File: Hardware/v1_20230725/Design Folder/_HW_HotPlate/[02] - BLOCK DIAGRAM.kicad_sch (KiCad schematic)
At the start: 0 parts

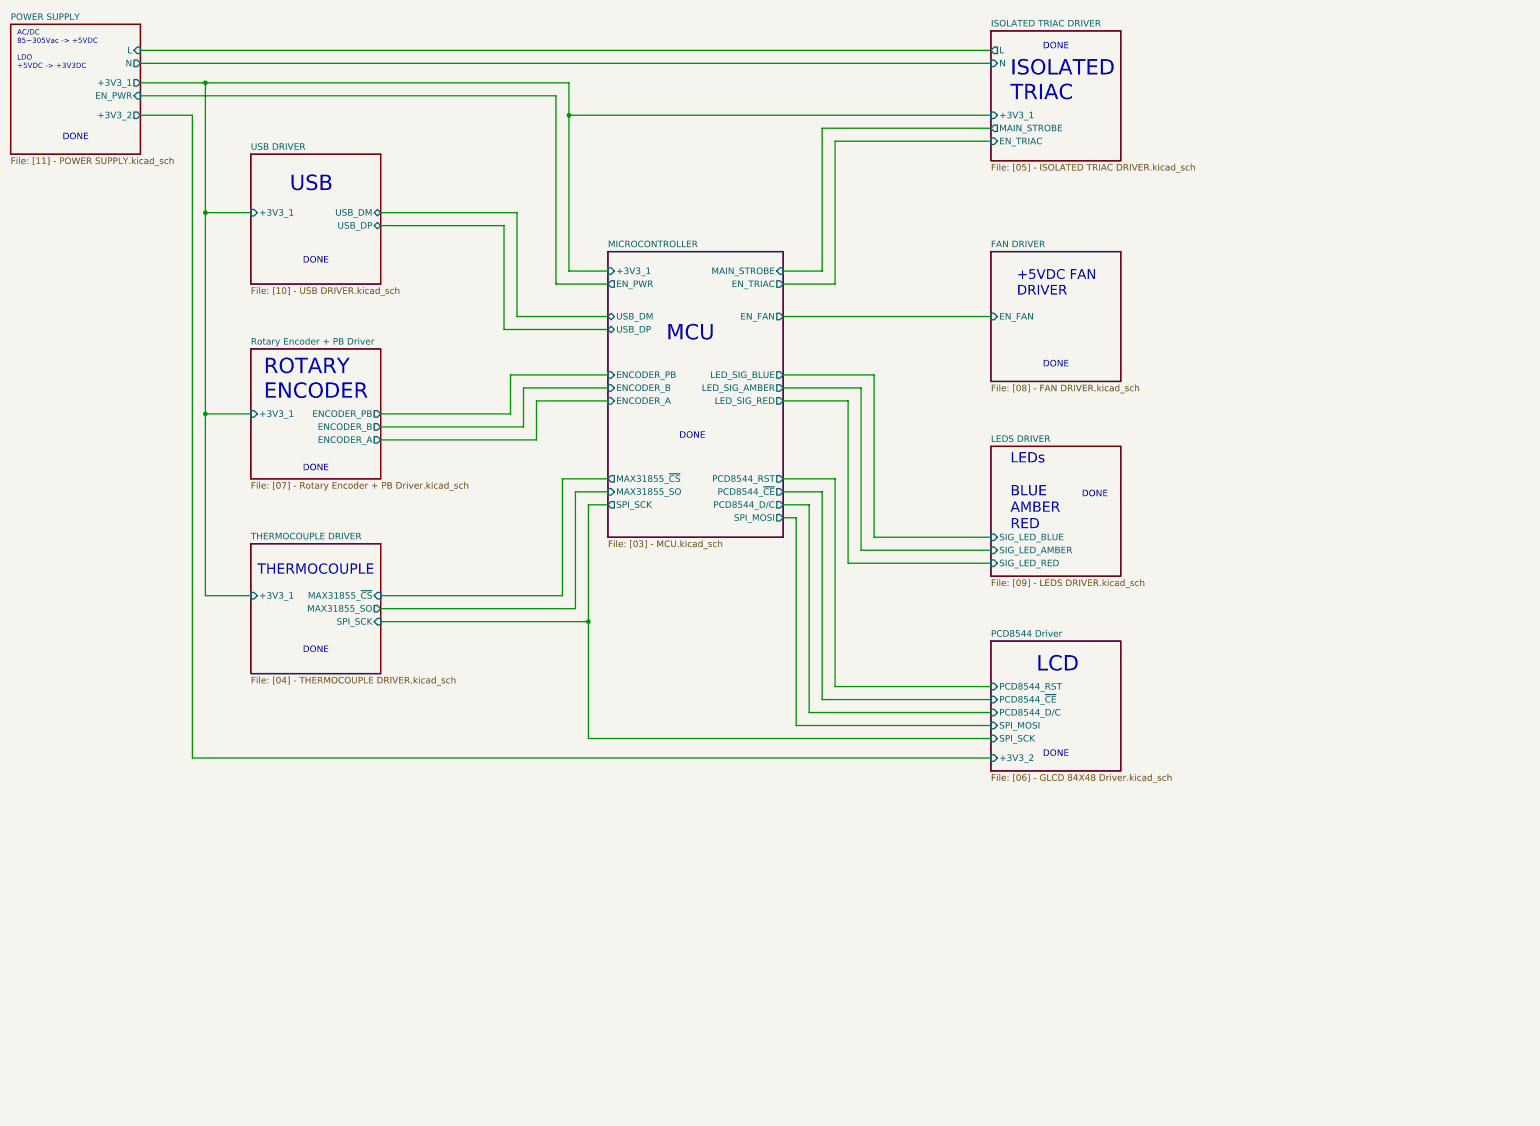
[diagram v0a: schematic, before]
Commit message: Updating hardware format structure
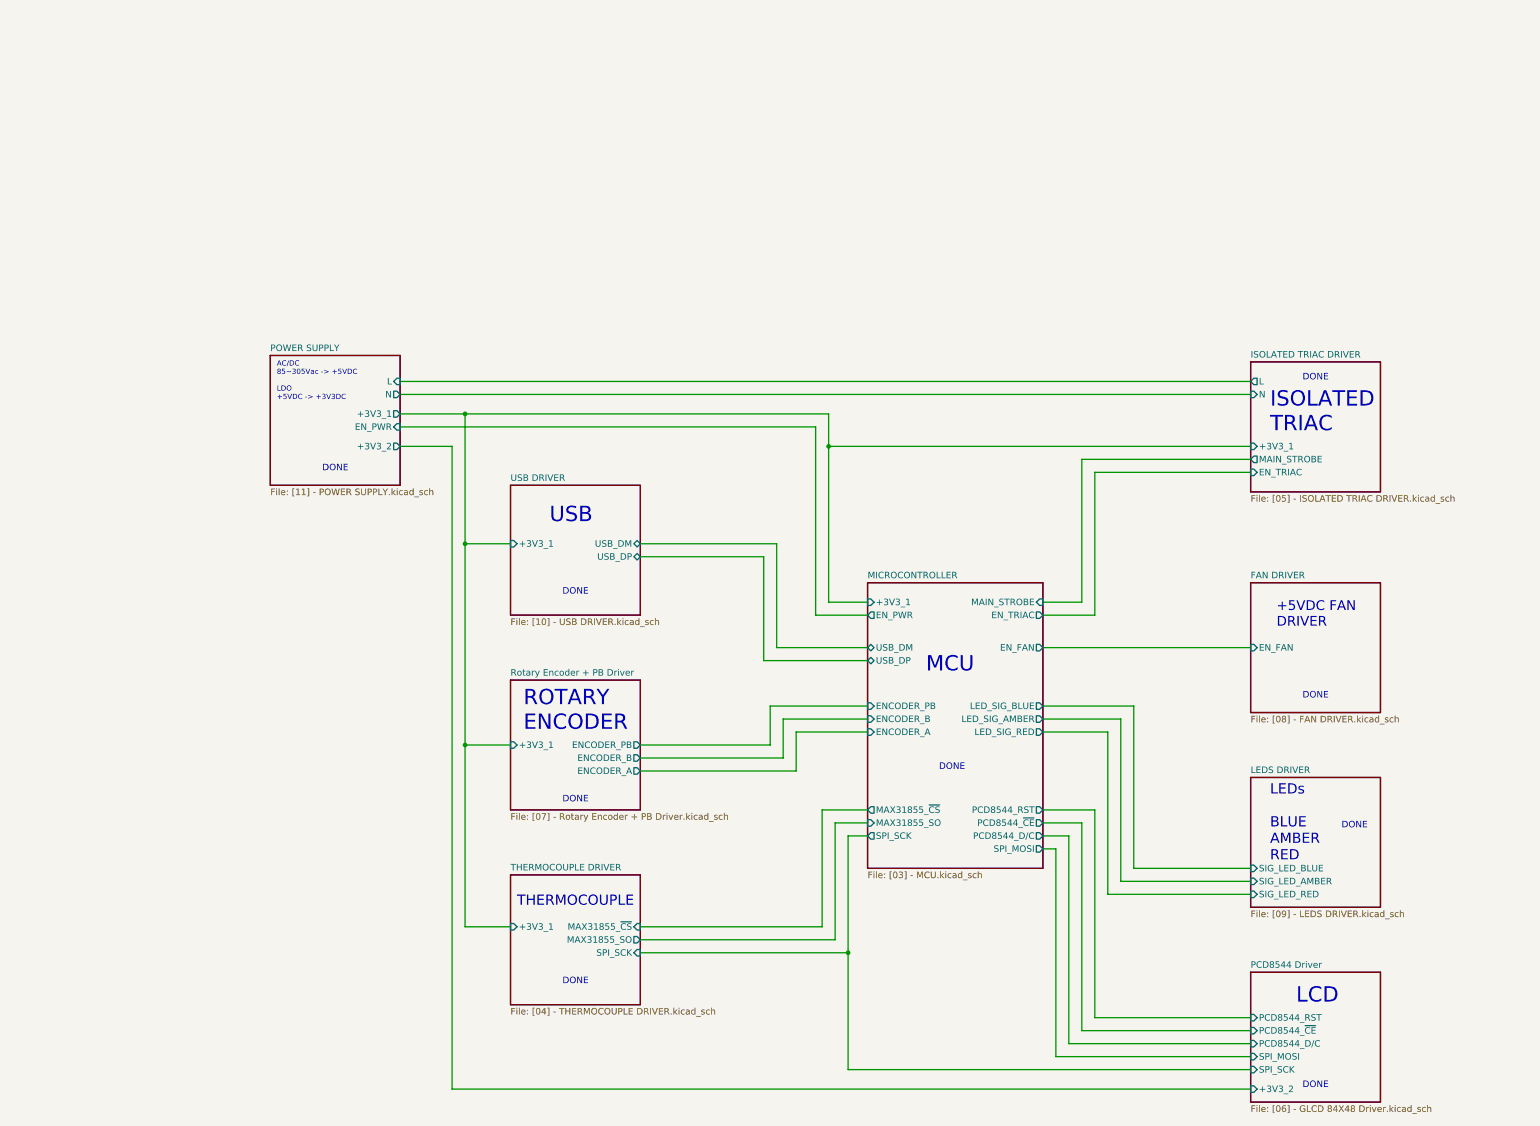
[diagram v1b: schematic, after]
